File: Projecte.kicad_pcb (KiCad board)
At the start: 4 copper layers, 107.1 x 75.3 mm, 56 parts, among them K1 A161CS12VDC.64, Q1 IRLZ34N, Q3 IRLZ34N, Q4 IRLZ34N, Q5 IRLZ34N, Q7 IRLZ34N, U1 PIC18F448-IP, U2 LM358, U3 R-786.5-0.5, U4 MCP2551-I-P, U5 AMS1117-3.3, U6 TXB0108PW, U7 LM7805_TO220, U8 MMC5883MA, Y1 Crystal

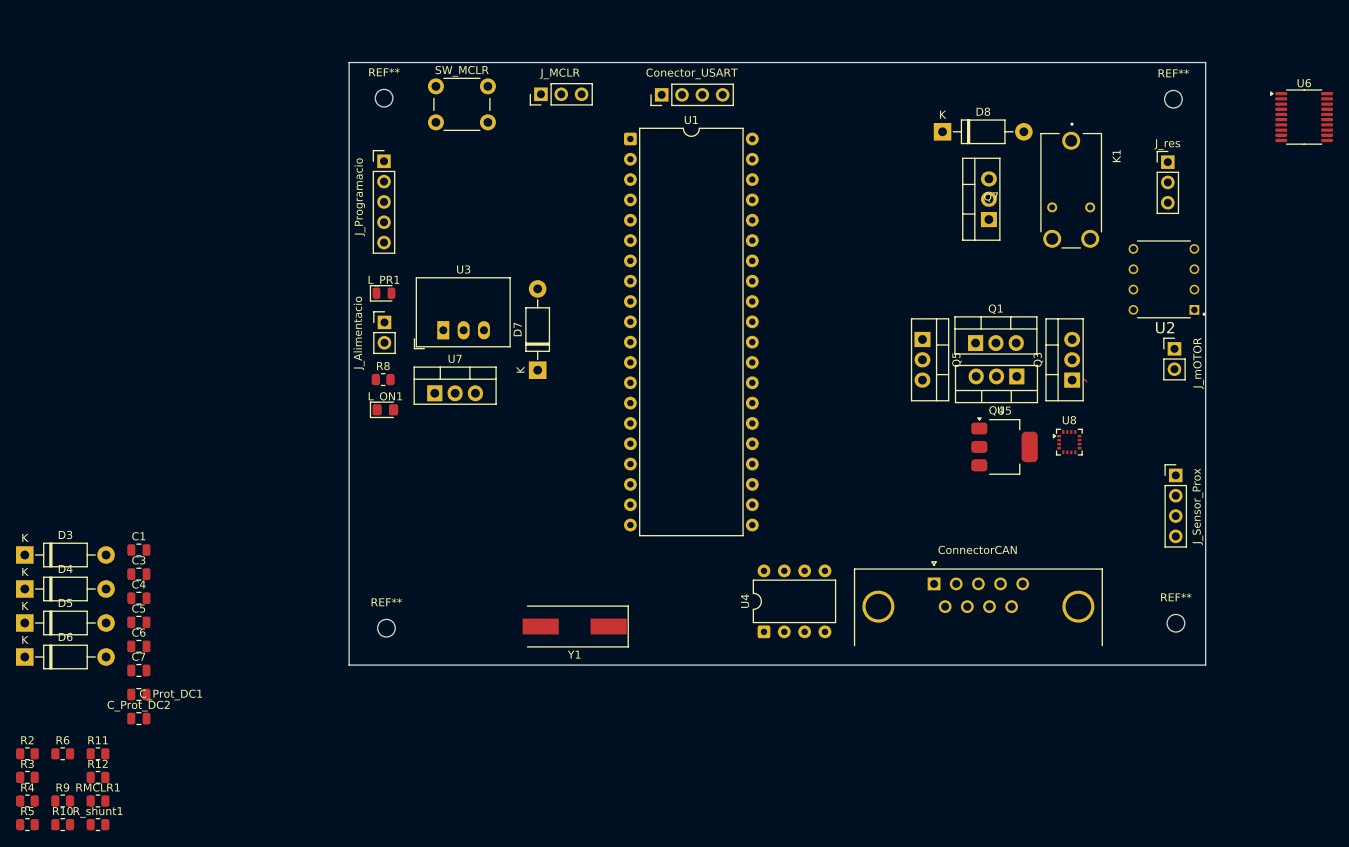
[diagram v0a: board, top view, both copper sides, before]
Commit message: Layout
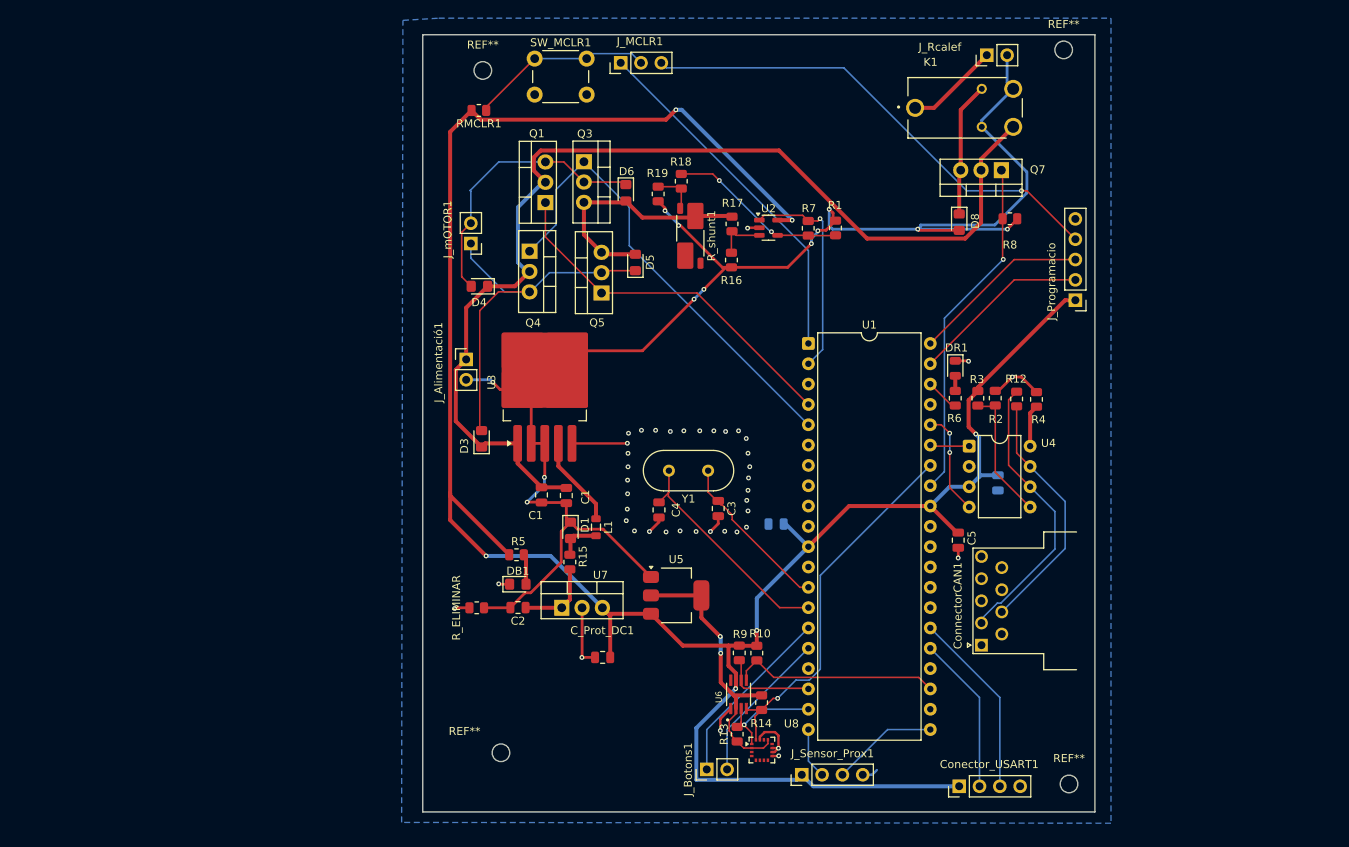
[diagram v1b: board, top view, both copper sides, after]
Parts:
- removed C_Prot_DC2: 0,33u, Capacitor_SMD:C_0805_2012Metric
- removed ConnectorCAN: DE9_Pins, Connector_Dsub:DSUB-9_Pins_Horizontal_P2.77x2.84mm_EdgePinOffset4.94mm_Housed_MountingHolesOffset4.94mm
- removed D7: D, Diode_THT:D_DO-41_SOD81_P10.16mm_Horizontal
- removed J_Alimentacio: Conn_01x02_Pin, Connector_PinHeader_2.54mm:PinHeader_1x02_P2.54mm_Vertical
- removed J_res: Conn_01x03_Pin, Connector_PinHeader_2.54mm:PinHeader_1x03_P2.54mm_Vertical
- added C1: 470u, Capacitor_SMD:C_0805_2012Metric, F.Cu at (112.0, 112.1)
- added C2: 20u, Capacitor_SMD:C_0805_2012Metric, F.Cu at (109.1, 126.2)
- added ConnectorCAN1: DE9_Pins, Connector_Dsub:DSUB-9_Pins_Horizontal_P2.77x2.54mm_EdgePinOffset9.40mm, F.Cu at (167.0, 130.9)
- added D1: Schttky, Diode_SMD:D_0805_2012Metric_Pad1.15x1.40mm_HandSolder, F.Cu at (115.7, 116.5)
- added J_Alimentació1: Conn_01x02_Pin, Connector_PinHeader_2.54mm:PinHeader_1x02_P2.54mm_Vertical, F.Cu at (102.6, 95.1)
- added J_Botons1: Conn_01x02_Pin, Connector_PinHeader_2.54mm:PinHeader_1x02_P2.54mm_Vertical, F.Cu at (132.7, 146.4)
- added J_Rcalef: Conn_01x02_Pin, Connector_PinHeader_2.54mm:PinHeader_1x02_P2.54mm_Vertical, F.Cu at (167.7, 57.1)
- added L1: L, Inductor_SMD:L_0805_2012Metric, F.Cu at (118.8, 116.1)
- added R1: 1k, Resistor_SMD:R_0805_2012Metric, F.Cu at (148.8, 78.7)
- added R13: R, Resistor_SMD:R_0805_2012Metric, F.Cu at (136.5, 142.0)
- added R14: R, Resistor_SMD:R_0805_2012Metric, F.Cu at (139.5, 138.0)
- added R15: R, Resistor_SMD:R_0805_2012Metric, F.Cu at (115.6, 120.5)
- added R16: 2k, Resistor_SMD:R_0805_2012Metric, F.Cu at (135.8, 82.7)
- added R17: 1k, Resistor_SMD:R_0805_2012Metric, F.Cu at (135.8, 78.2)
- added R18: 1k, Resistor_SMD:R_0805_2012Metric, F.Cu at (129.5, 72.9)
- added R19: 1k, Resistor_SMD:R_0805_2012Metric, F.Cu at (126.6, 74.5)
- added R7: 2k, Resistor_SMD:R_0805_2012Metric, F.Cu at (145.4, 78.8)
- C6, C7: moved to B.Cu
- D3, D4, D5, D6, D8: footprint Diode_THT:D_DO-41_SOD81_P10.16mm_Horizontal -> Diode_SMD:D_0805_2012Metric_Pad1.15x1.40mm_HandSolder
- R10, R9: value 10k -> R
- R_shunt1: value 0.005 -> 0.005R; footprint Resistor_SMD:R_0805_2012Metric -> Resistor_SMD:R_Shunt_Vishay_WSK2512_6332Metric_T2.21mm
- U2: value LM358 -> OPA336Nx; footprint Library:LM358 -> Package_TO_SOT_SMD:SOT-23-5
- U3: value R-786.5-0.5 -> LM2596S-3.3; footprint Converter_DCDC:Converter_DCDC_RECOM_R-78E-0.5_THT -> Package_TO_SOT_SMD:TO-263-5_TabPin3
- U6: value TXB0108PW -> PCA9306; footprint Package_SO:TSSOP-20_4.4x6.5mm_P0.65mm -> Library:PCA
- Y1: footprint Crystal:Crystal_SMD_HC49-SD -> Crystal:Crystal_HC18-U_Vertical
- moved R4 135.8 mm to (173.9, 100.1), turned to -90 degrees
- moved R3 129.9 mm to (168.8, 100.0), turned to 90 degrees
- moved R2 126.8 mm to (166.6, 100.0), turned to -90 degrees
- moved R12 124.2 mm to (171.4, 100.1), turned to -90 degrees
- moved R6 120.1 mm to (163.8, 100.0), turned to -90 degrees
- moved C6 109.3 mm to (169.1, 110.6), turned to -90 degrees
- moved R_shunt1 104.4 mm to (130.6, 79.7), turned to -90 degrees
- moved C5 102.9 mm to (164.1, 117.7), turned to -90 degrees
- moved U6 101.0 mm to (136.7, 137.0), turned to 90 degrees
- moved RMCLR1 98.6 mm to (104.2, 64.0), turned to 180 degrees
- moved D6 94.9 mm to (122.6, 74.3), turned to -90 degrees
- moved Conector_USART1 94.1 mm to (164.2, 148.5)
- moved R10 89.4 mm to (138.9, 131.8), turned to -90 degrees
- moved J_mOTOR1 88.9 mm to (103.2, 80.7), turned to 180 degrees
- moved D5 88.6 mm to (123.8, 83.0), turned to 90 degrees
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- renumbered Conector_USART to Conector_USART1, L_ON1 to DB1, L_PR1 to DR1, J_MCLR to J_MCLR1, J_Sensor_Prox to J_Sensor_Prox1, J_mOTOR to J_mOTOR1, R11 to R_ELIMINAR, SW_MCLR to SW_MCLR1
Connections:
- net /CORRENT! renamed /corrent
- net Net-(L_ON1-A) renamed /V_LED_ON
- net Net-(L_PR1-A) renamed /V_LED_XIP
- net Net-(U4-Rs) renamed /RsU4
- R10 pad 1: /Vcc -> VCC
- R10 pad 2: /apagar? -> /SDA
- R8 pad 2: unconnected-(R8-Pad2) -> GNDPWR
- R9 pad 1: /Vcc_3.3V -> VCC
- R9 pad 2: /final_carrera -> /SCL
- R_shunt1 pad 2: GNDPWR -> Net-(R18-Pad2)
- U1 pad 19: /Datos_i2c -> /SCL_S
- U1 pad 34: /apagar? -> /SDA_S
- U2 pad 2: GNDPWR -> GND
- U2 pad 3: /shunt -> Net-(U2-+)
- U2 pad 4: (no net) -> /V-s
- U2 pad 5: (no net) -> VCC
- U3 pad 3: Net-(D7-A) -> GNDPWR
- U5 pad 3: /Vcc -> VCC
- U6 pad 1: /SCL -> GND
- U6 pad 3: /SDA -> /SCL_S
- U6 pad 4: unconnected-(U6-A3-Pad4) -> /SDA_S
- U6 pad 5: unconnected-(U6-A4-Pad5) -> /SDA
- U6 pad 6: unconnected-(U6-A5-Pad6) -> /SCL
- U6 pad 7: unconnected-(U6-A6-Pad7) -> VCC
- U6 pad 8: /final_carrera -> unconnected-(U6-EN-Pad8)
- U7 pad 1: Net-(D7-A) -> /7V
- U8 pad 15: /final_carrera -> GND
- U8 pad 16: /i2c_nivellat -> /SDA_S
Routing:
- net VCC: track 0.00 -> 296.5 mm, vias 0 -> 6
- net GNDPWR: track 0.00 -> 207.5 mm, vias 0 -> 12
- net +12V: track 0.00 -> 136.2 mm
- net /Vpp: track 0.00 -> 60.9 mm, vias 0 -> 1
- net /Pujar: track 0.37 -> 58.5 mm
- net /M+: track 0.00 -> 47.5 mm
- net /SDA_S: track 0.00 -> 46.7 mm, vias 0 -> 1
- net GND: track 0.00 -> 46.4 mm, vias 0 -> 42
- net /Baixar: track 0.00 -> 45.8 mm
- net /MCLR: track 0.00 -> 44.8 mm
- net /R_on: track 0.00 -> 43.3 mm, vias 0 -> 1
- net /Canl: track 0.00 -> 36.0 mm
- net /Vcc_3.3V: track 0.00 -> 35.5 mm, vias 0 -> 2
- net /M-: track 0.00 -> 35.1 mm
- net /Canh: track 0.00 -> 31.5 mm
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- added copper zone on B.Cu, net GND
- removed copper zone on In2.Cu, net GND
- removed copper zone on In1.Cu, net VCC
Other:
- board size 107.1 x 75.3 mm -> 84 x 97.2 mm
- copper layers 4 -> 2
